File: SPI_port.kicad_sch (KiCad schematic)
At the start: 5 parts, among them J12 Conn_01x06_Female

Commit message: pcb is in progress, finishing H-bridge layout
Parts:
- D100, D101, D97, D98: footprint Diode_SMD:D_SMB -> _Diodes:SM2T3V3A
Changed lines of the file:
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@@
       (effects (font (size 1.27 1.27)) (justify left) hide)
     )
-    (property "Footprint" "Diode_SMD:D_SMB" (id 2) (at 144.78 102.87 0)
+    (property "Footprint" "_Diodes:SM2T3V3A" (id 2) (at 144.78 102.87 0)
       (effects (font (size 1.27 1.27)) hide)
     )
@@
       (effects (font (size 1.27 1.27)) (justify left) hide)
     )
-    (property "Footprint" "Diode_SMD:D_SMB" (id 2) (at 137.16 102.87 0)
+    (property "Footprint" "_Diodes:SM2T3V3A" (id 2) (at 137.16 102.87 0)
       (effects (font (size 1.27 1.27)) hide)
     )
@@
       (effects (font (size 1.27 1.27)) (justify left) hide)
     )
-    (property "Footprint" "Diode_SMD:D_SMB" (id 2) (at 140.97 102.87 0)
+    (property "Footprint" "_Diodes:SM2T3V3A" (id 2) (at 140.97 102.87 0)
       (effects (font (size 1.27 1.27)) hide)
     )
@@
       (effects (font (size 1.27 1.27)) (justify left))
     )
-    (property "Footprint" "Diode_SMD:D_SMB" (id 2) (at 133.35 102.87 0)
+    (property "Footprint" "_Diodes:SM2T3V3A" (id 2) (at 133.35 102.87 0)
       (effects (font (size 1.27 1.27)) hide)
     )

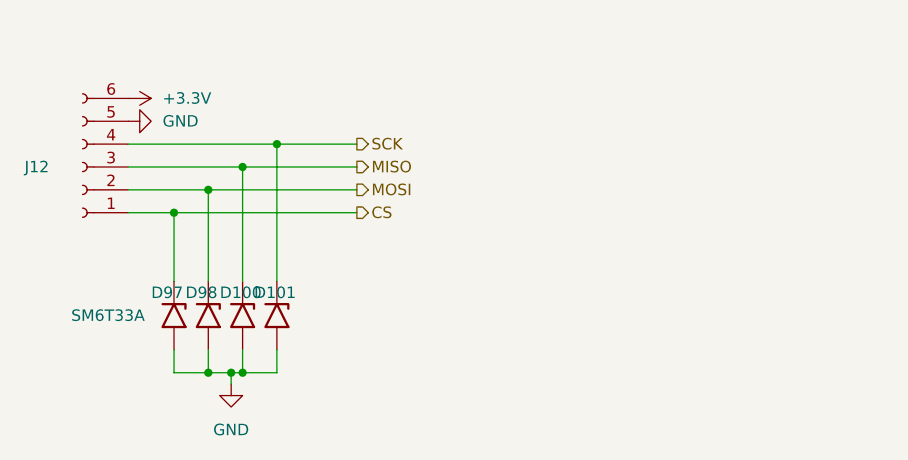
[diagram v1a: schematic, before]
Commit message: project finished before changes
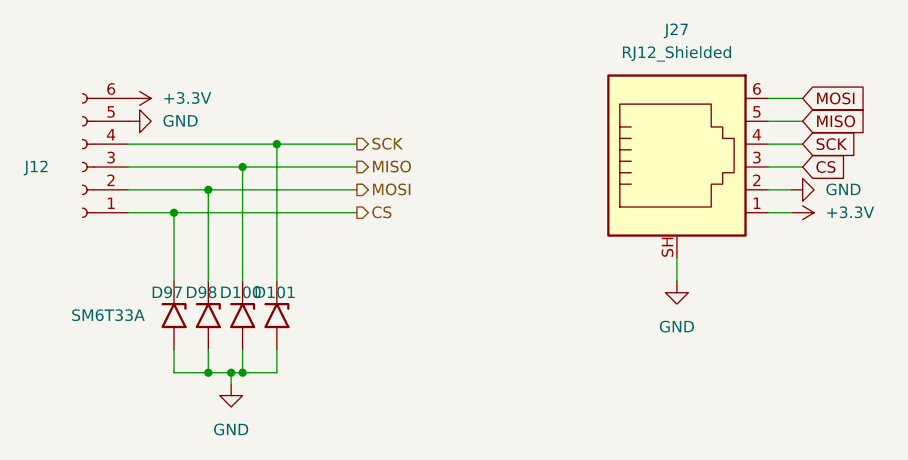
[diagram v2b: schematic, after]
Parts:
- added J27: RJ12_Shielded, _Connectors:RJ12_Shielded, symbol _Connectors:RJ12_Shielded
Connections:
- net +3V3: now also J27.1
- net CS: now also J27.3
- net GND: now also J27.2, J27.SH
- net MISO: now also J27.5
- net MOSI: now also J27.6
- net SCK: now also J27.4
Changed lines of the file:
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@@
+    (stroke (width 0) (type default) (color 0 0 0 0))
+  )
+  (wire (pts (xy 204.47 83.82) (xy 208.28 83.82))
     (stroke (width 0) (type default) (color 0 0 0 0))
   )
@@
     (stroke (width 0) (type default) (color 0 0 0 0))
   )
+  (wire (pts (xy 204.47 78.74) (xy 208.28 78.74))
+    (stroke (width 0) (type default) (color 0 0 0 0))
+  )
   (wire (pts (xy 158.75 91.44) (xy 138.43 91.44))
     (stroke (width 0) (type default) (color 0 0 0 0))
@@
     (stroke (width 0) (type default) (color 0 0 0 0))
   )
+  (wire (pts (xy 204.47 88.9) (xy 207.01 88.9))
+    (stroke (width 0) (type default) (color 0 0 0 0))
+  )
   (wire (pts (xy 146.05 106.68) (xy 146.05 109.22))
     (stroke (width 0) (type default) (color 0 0 0 0))
   )
+  (wire (pts (xy 194.31 96.52) (xy 194.31 99.06))
+    (stroke (width 0) (type default) (color 0 0 0 0))
+  )
   (wire (pts (xy 144.78 109.22) (xy 144.78 110.49))
     (stroke (width 0) (type default) (color 0 0 0 0))
@@
     (stroke (width 0) (type default) (color 0 0 0 0))
   )
+  (wire (pts (xy 204.47 91.44) (xy 207.01 91.44))
+    (stroke (width 0) (type default) (color 0 0 0 0))
+  )
   (wire (pts (xy 149.86 99.06) (xy 149.86 83.82))
     (stroke (width 0) (type default) (color 0 0 0 0))
@@
     (stroke (width 0) (type default) (color 0 0 0 0))
   )
+  (wire (pts (xy 204.47 81.28) (xy 208.28 81.28))
+    (stroke (width 0) (type default) (color 0 0 0 0))
+  )
   (wire (pts (xy 146.05 109.22) (xy 149.86 109.22))
     (stroke (width 0) (type default) (color 0 0 0 0))
   )
+  (wire (pts (xy 204.47 86.36) (xy 208.28 86.36))
+    (stroke (width 0) (type default) (color 0 0 0 0))
+  )
+  (global_label "SCK" (shape input) (at 208.28 83.82 0) (fields_autoplaced)
+    (effects (font (size 1.27 1.27)) (justify left))
+    (property "Intersheet References" "${INTERSHEET_REFS}" (id 0) (at 214.4426 83.7406 0)
+      (effects (font (size 1.27 1.27)) (justify left) hide)
+    )
+  )
+  (global_label "MISO" (shape input) (at 208.28 81.28 0) (fields_autoplaced)
+    (effects (font (size 1.27 1.27)) (justify left))
+    (property "Intersheet References" "${INTERSHEET_REFS}" (id 0) (at 215.2893 81.2006 0)
+      (effects (font (size 1.27 1.27)) (justify left) hide)
+    )
+  )
+  (global_label "MOSI" (shape input) (at 208.28 78.74 0) (fields_autoplaced)
+    (effects (font (size 1.27 1.27)) (justify left))
+    (property "Intersheet References" "${INTERSHEET_REFS}" (id 0) (at 215.2893 78.6606 0)
+      (effects (font (size 1.27 1.27)) (justify left) hide)
+    )
+  )
+  (global_label "CS" (shape input) (at 208.28 86.36 0) (fields_autoplaced)
+    (effects (font (size 1.27 1.27)) (justify left))
+    (property "Intersheet References" "${INTERSHEET_REFS}" (id 0) (at 213.1726 86.2806 0)
+      (effects (font (size 1.27 1.27)) (justify left) hide)
+    )
+  )
   (hierarchical_label "MISO" (shape output) (at 158.75 86.36 0)
     (effects (font (size 1.27 1.27)) (justify left))
@@
     )
     (property "Datasheet" "" (id 3) (at 133.35 78.74 0)
+      (effects (font (size 1.27 1.27)) hide)
+    )
+    (pin "1")
+  )
+  (symbol (lib_id "power:+3.3V") (at 207.01 91.44 270) (unit 1)
+    (in_bom yes) (on_board yes) (fields_autoplaced)
+    (property "Reference" "#PWR0206" (id 0) (at 203.2 91.44 0)
+      (effects (font (size 1.27 1.27)) hide)
+    )
+    (property "Value" "+3.3V" (id 1) (at 210.82 91.4399 90)
+      (effects (font (size 1.27 1.27)) (justify left))
+    )
+    (property "Footprint" "" (id 2) (at 207.01 91.44 0)
+      (effects (font (size 1.27 1.27)) hide)
+    )
+    (property "Datasheet" "" (id 3) (at 207.01 91.44 0)
       (effects (font (size 1.27 1.27)) hide)
     )
@@
     (pin "1")
   )
+  (symbol (lib_id "power:GND") (at 207.01 88.9 90) (unit 1)
+    (in_bom yes) (on_board yes) (fields_autoplaced)
+    (property "Reference" "#PWR0164" (id 0) (at 213.36 88.9 0)
+      (effects (font (size 1.27 1.27)) hide)
+    )
+    (property "Value" "GND" (id 1) (at 210.82 88.8999 90)
+      (effects (font (size 1.27 1.27)) (justify right))
+    )
+    (property "Footprint" "" (id 2) (at 207.01 88.9 0)
+      (effects (font (size 1.27 1.27)) hide)
+    )
+    (property "Datasheet" "" (id 3) (at 207.01 88.9 0)
+      (effects (font (size 1.27 1.27)) hide)
+    )
+    (pin "1")
+  )
   (symbol (lib_id "Diode:SM6T33A") (at 142.24 102.87 270) (unit 1)
     (in_bom yes) (on_board yes)
@@
     (pin "1")
     (pin "2")
+  )
+  (symbol (lib_id "power:GND") (at 194.31 99.06 0) (unit 1)
+    (in_bom yes) (on_board yes) (fields_autoplaced)
+    (property "Reference" "#PWR0157" (id 0) (at 194.31 105.41 0)
+      (effects (font (size 1.27 1.27)) hide)
+    )
+    (property "Value" "GND" (id 1) (at 194.31 104.14 0))
+    (property "Footprint" "" (id 2) (at 194.31 99.06 0)
+      (effects (font (size 1.27 1.27)) hide)
+    )
+    (property "Datasheet" "" (id 3) (at 194.31 99.06 0)
+      (effects (font (size 1.27 1.27)) hide)
+    )
+    (pin "1")
   )
   (symbol (lib_id "power:GND") (at 133.35 81.28 90) (unit 1)
@@
     (pin "2")
   )
+  (symbol (lib_id "_Connectors:RJ12_Shielded") (at 194.31 86.36 0) (unit 1)
+    (in_bom yes) (on_board yes) (fields_autoplaced)
+    (property "Reference" "J27" (id 0) (at 194.31 71.12 0))
+    (property "Value" "RJ12_Shielded" (id 1) (at 194.31 73.66 0))
+    (property "Footprint" "_Connectors:RJ12_Shielded" (id 2) (at 186.69 102.87 0)
+      (effects (font (size 1.27 1.27)) hide)
+    )
+    (property "Datasheet" "https://docs.rs-online.com/f10d/0900766b813030b0.pdf" (id 3) (at 201.93 100.33 0)
+      (effects (font (size 1.27 1.27)) hide)
+    )
+    (pin "1")
+    (pin "2")
+    (pin "3")
+    (pin "4")
+    (pin "5")
+    (pin "6")
+    (pin "SH")
+  )
 )
